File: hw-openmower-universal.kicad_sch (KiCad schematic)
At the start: 25 parts

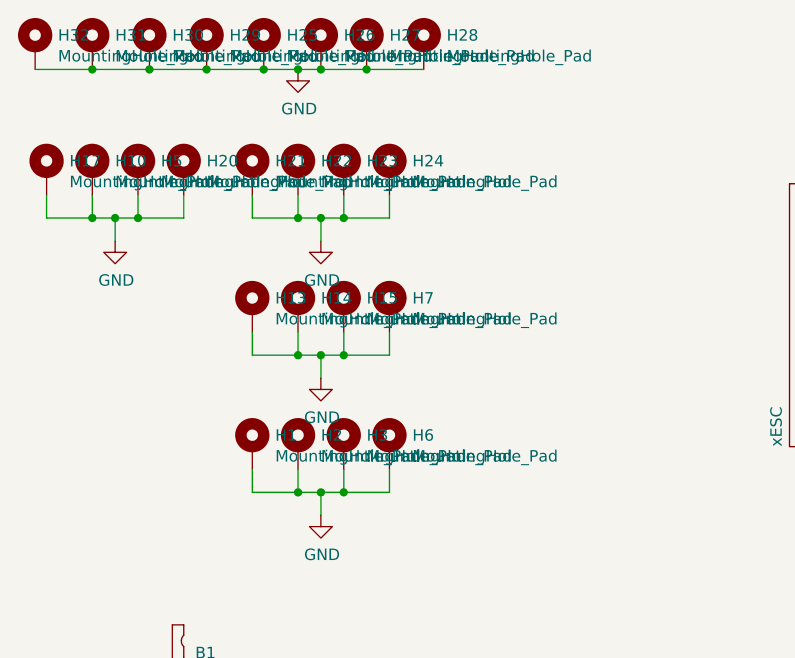
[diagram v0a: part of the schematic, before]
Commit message: Further routing progress
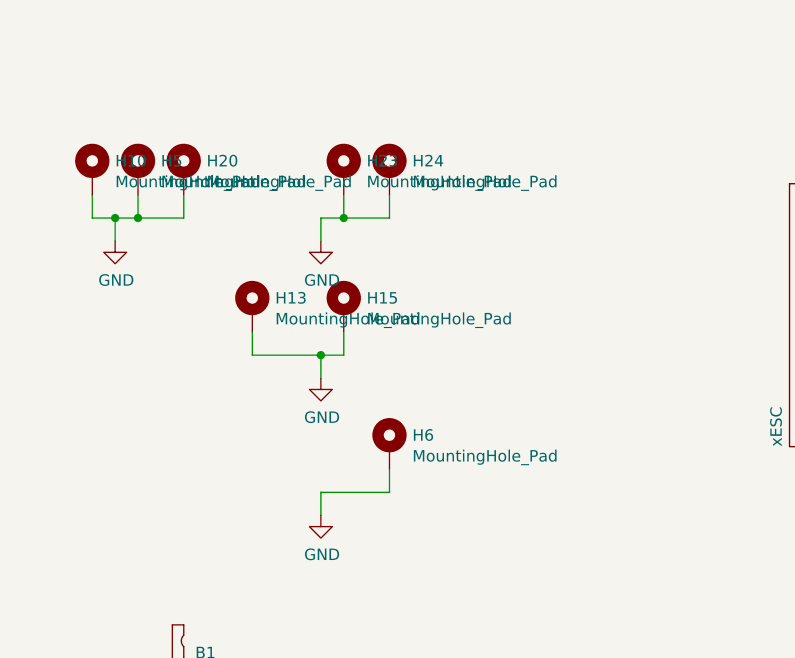
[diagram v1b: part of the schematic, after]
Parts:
- removed H1, H14, H17, H2, H21, H22, H25, H26, H27, H28, H29, H3, H30, H31, H32, H7: MountingHole_Pad, MountingHole:MountingHole_4.3mm_M4_Pad_Via, symbol Mechanical:MountingHole_Pad
